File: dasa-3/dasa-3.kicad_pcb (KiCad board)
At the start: 2 copper layers, 31.5 x 63.5 mm, 12 parts, among them J1 DB9_Male, J2 AVR-ISP-10, J3 AVR-ISP-6, Q1 BC546

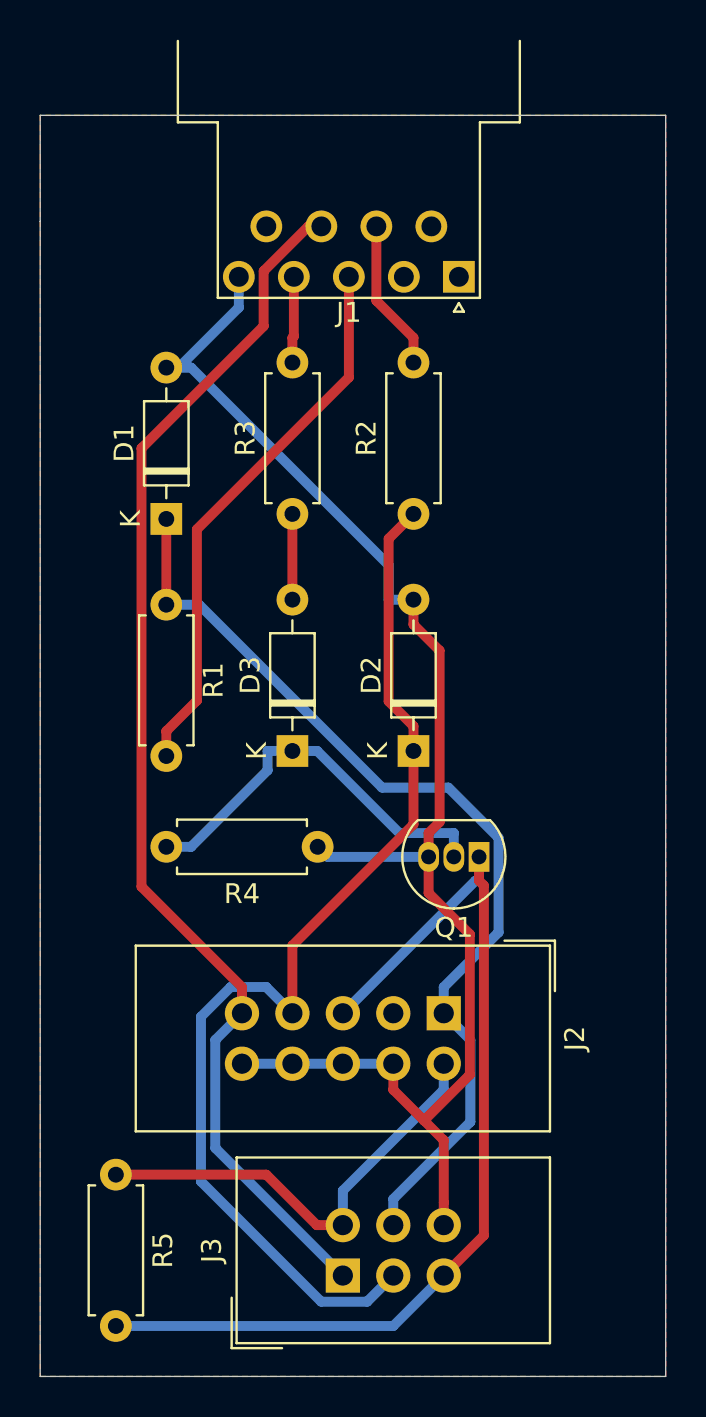
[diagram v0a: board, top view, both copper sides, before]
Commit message: update: update project files
Signed-off-by: Paweł Sobótka <48721262935pl@gmail.com>
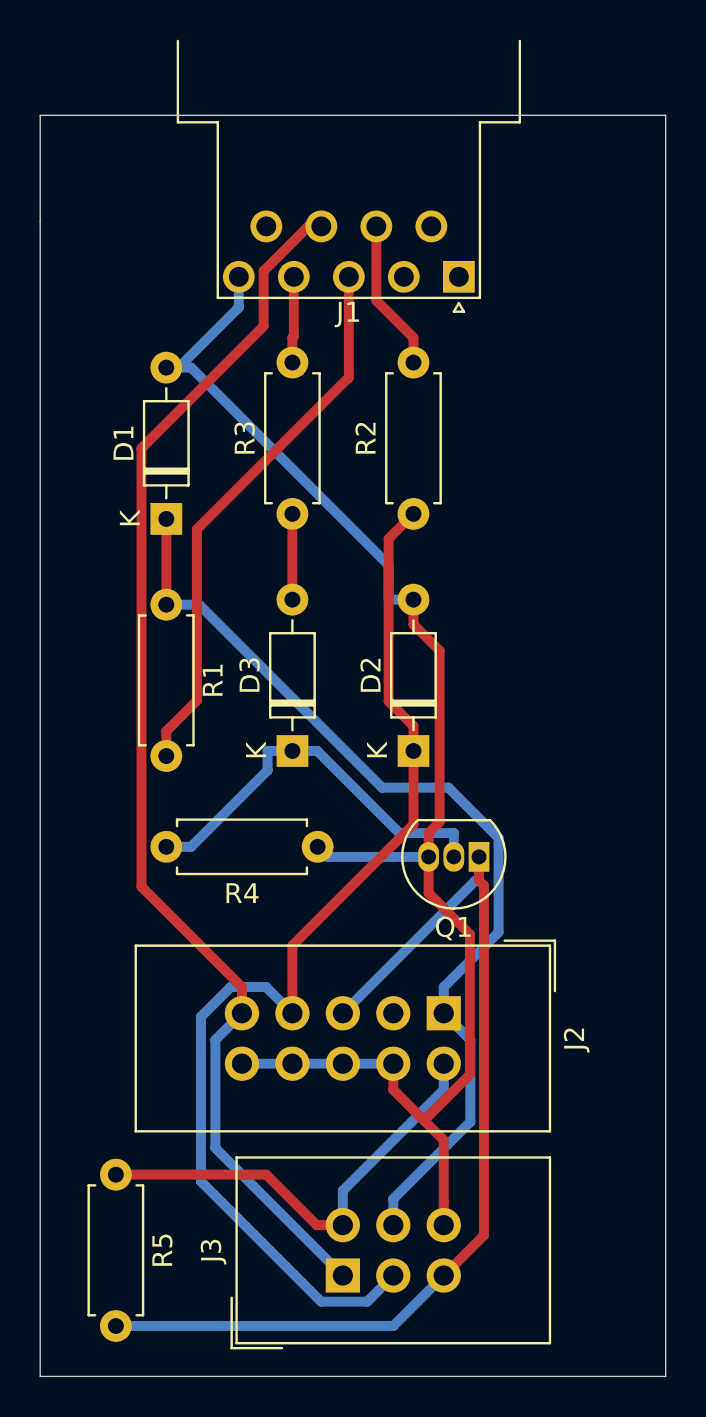
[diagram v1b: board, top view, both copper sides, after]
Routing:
- removed copper zone on F.Cu, net GND
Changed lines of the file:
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@@
-(kicad_pcb (version 20171130) (host pcbnew 5.1.2-1.fc30)
+(kicad_pcb (version 20171130) (host pcbnew 5.1.4-3.fc30)
   (general
     (thickness 1.6)
-    (drawings 7)
+    (drawings 8)
     (tracks 97)
     (zones 0)
@@
   (page A4)
   (title_block
-    (title "avr dasa-3 programmer PCB")
-    (date 2019-07-21)
-    (rev 0.5)
+    (title "AVR dasa-3 programmer PCB layout")
+    (date 2019-09-20)
+    (rev 1.0)
     (company "mgr inż. Paweł Sobótka")
+    (comment 1 "GNU GPLv3")
+    (comment 2 "Device AVR Serial Adapter")
   )
   (layers
@@
       (drillshape 0)
       (scaleselection 1)
-      (outputdirectory "grbv/"))
+      (outputdirectory "gerbv/"))
   )
   (net 0 "")
@@
     )
   )
+  (target plus (at 118.9609 87.85352) (size 5) (width 0.05) (layer Edge.Cuts))
   (gr_text "avr \"dasa-3\" programmer" (at 144.018 79.248 90) (layer Dwgs.User)
     (effects (font (size 1 1) (thickness 0.15)))
@@
   (segment (start 120.396 108.966) (end 134.366 108.966) (width 0.5) (layer B.Cu) (net 16))
   (segment (start 134.366 108.966) (end 136.906 106.426) (width 0.5) (layer B.Cu) (net 16))
-  (zone (net 1) (net_name GND) (layer F.Cu) (hatch edge 0.508)
-    (connect_pads (clearance 0.508))
-    (min_thickness 0.254)
-    (fill yes (arc_segments 32) (thermal_gap 0.508) (thermal_bridge_width 0.508) (smoothing chamfer) (radius 3))
-    (polygon
-      (pts
-        (xy 116.586 48.006) (xy 116.586 111.506) (xy 148.082 111.506) (xy 148.082 48.006)
-      )
-    )
-  )
 )
